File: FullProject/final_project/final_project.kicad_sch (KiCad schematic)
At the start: 46 parts, among them J1 Conn_WallSocket, J2 Weight Sensor Connector, J3 PIR Array Connector 01, J4 PIR Array Connector 02, J5 PIR Array Connector 03, J6 pH Sensor Connector, J7 Keypad Connector, J8 LCD Connector, J9 Conn_01x02_Female, M1 Motor_DC, M2 Motor_Servo, Q1 2N4403, U1 L7805, U2 LM7809_TO220, U3 LM7812_TO220, U4 ATmega32A-P, U5 L293D, U6 SIM900, U7 DS3232M, U8 PCF8574

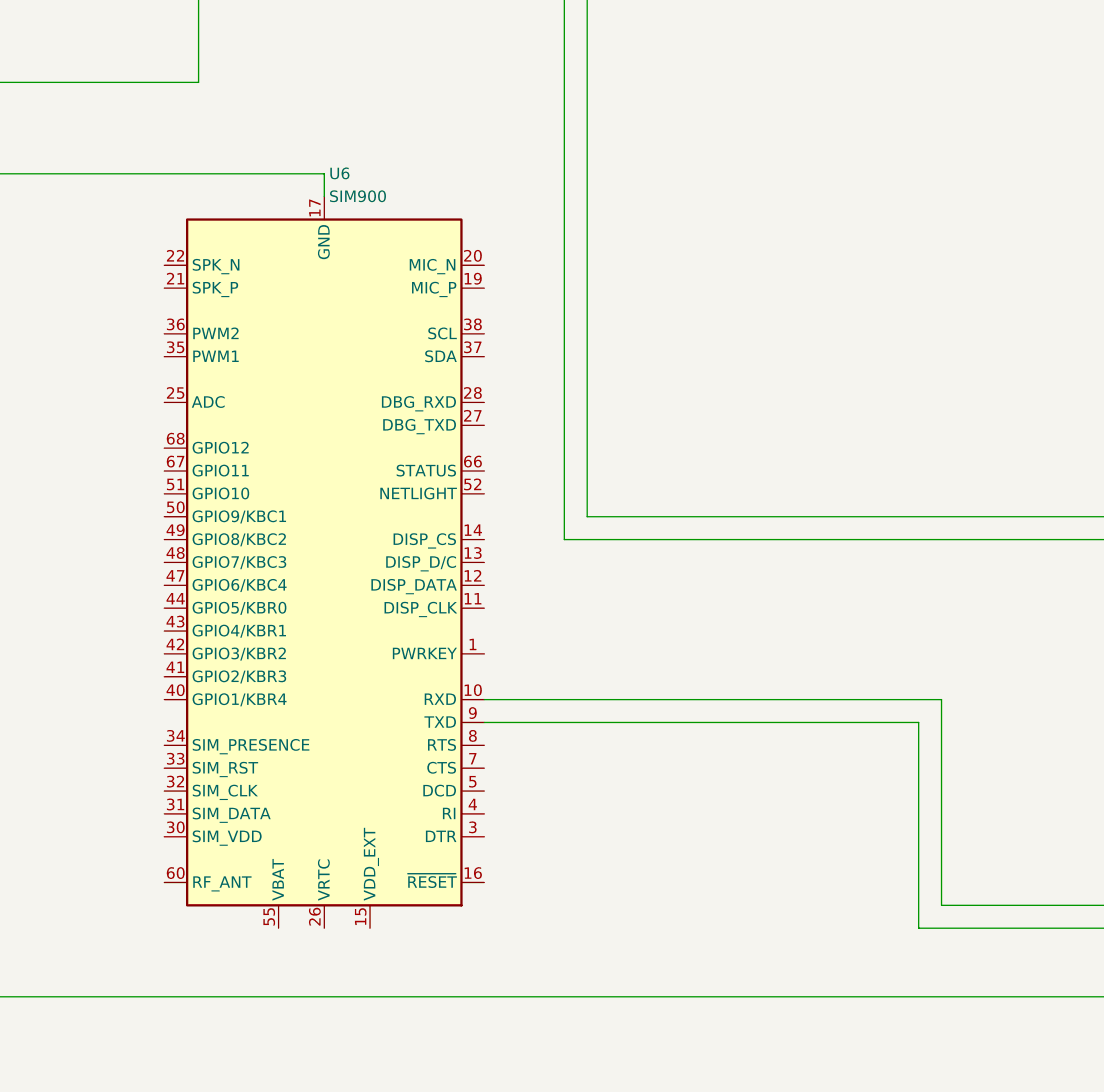
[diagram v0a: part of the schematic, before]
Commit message: add
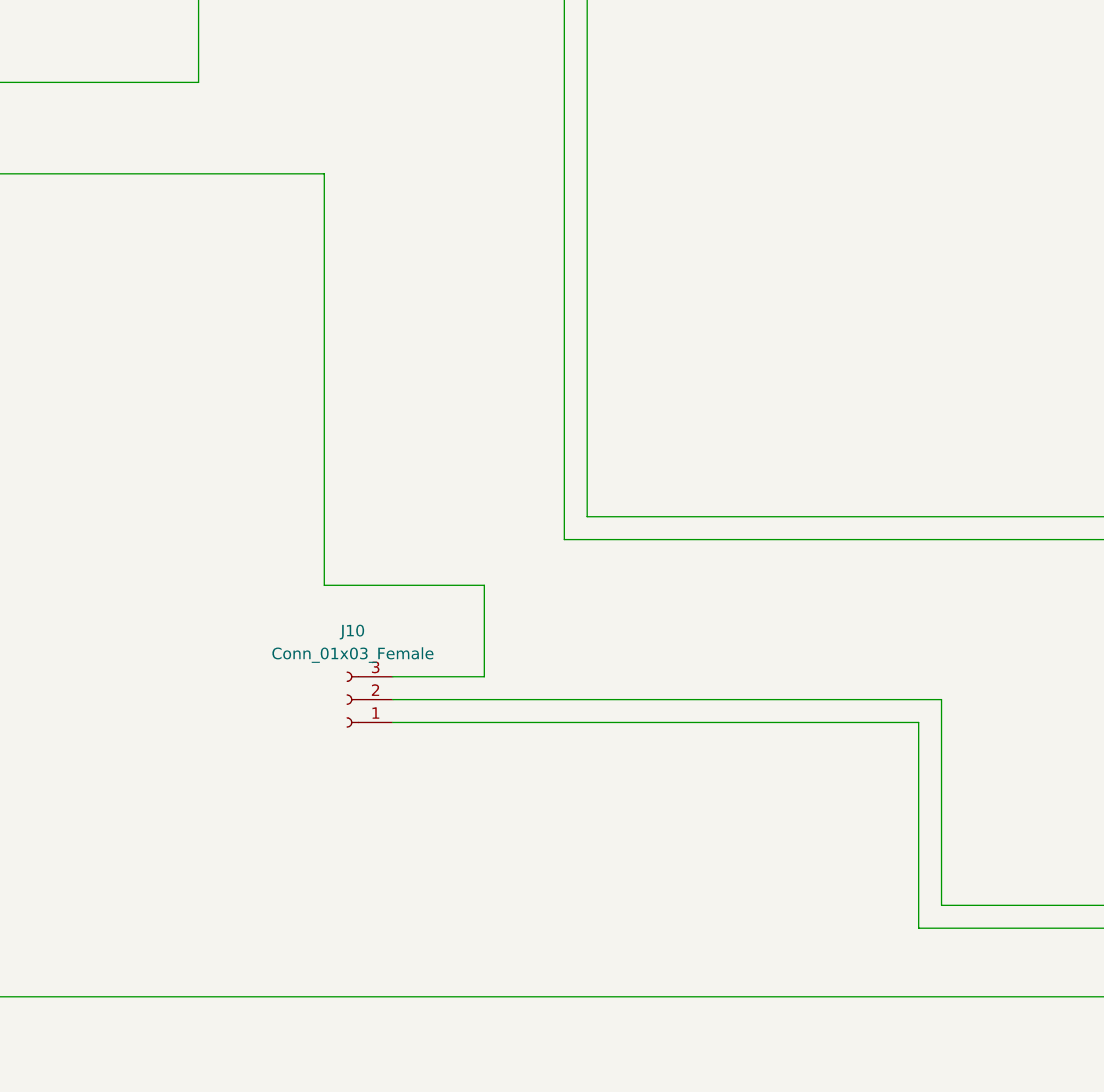
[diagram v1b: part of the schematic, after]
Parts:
- removed U6: SIM900, RF_GSM:SIMCom_SIM900, symbol RF_GSM:SIM900
- added J10: Conn_01x03_Female, Connector_PinSocket_2.54mm:PinSocket_1x03_P2.54mm_Vertical, symbol Connector:Conn_01x03_Female
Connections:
- net at BZ1.2 (+), C1.2, C2.1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: now also J10.3 (Pin_3)
- net at U4.15 (PD1): now also J10.2 (Pin_2)
- net at U4.14 (PD0): now also J10.1 (Pin_1)
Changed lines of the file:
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@@
     (stroke (width 0) (type default) (color 0 0 0 0))
   )
-  (wire (pts (xy 104.14 186.69) (xy 152.4 186.69))
+  (wire (pts (xy 93.98 186.69) (xy 152.4 186.69))
     (stroke (width 0) (type default) (color 0 0 0 0))
   )
@@
     (stroke (width 0) (type default) (color 0 0 0 0))
   )
-  (wire (pts (xy 104.14 184.15) (xy 154.94 184.15))
+  (wire (pts (xy 93.98 184.15) (xy 154.94 184.15))
     (stroke (width 0) (type default) (color 0 0 0 0))
   )
@@
     (stroke (width 0) (type default) (color 0 0 0 0))
   )
+  (wire (pts (xy 104.14 181.61) (xy 93.98 181.61))
+    (stroke (width 0) (type default) (color 0 0 0 0))
+  )
   (wire (pts (xy 113.03 166.37) (xy 175.26 166.37))
     (stroke (width 0) (type default) (color 0 0 0 0))
@@
     (stroke (width 0) (type default) (color 0 0 0 0))
   )
-  (wire (pts (xy 86.36 125.73) (xy 86.36 128.27))
-    (stroke (width 0) (type default) (color 0 0 0 0))
-  )
   (wire (pts (xy 234.95 184.15) (xy 228.6 184.15))
     (stroke (width 0) (type default) (color 0 0 0 0))
@@
     (stroke (width 0) (type default) (color 0 0 0 0))
   )
+  (wire (pts (xy 86.36 125.73) (xy 86.36 171.45))
+    (stroke (width 0) (type default) (color 0 0 0 0))
+  )
   (wire (pts (xy 292.1 224.79) (xy 248.92 224.79))
     (stroke (width 0) (type default) (color 0 0 0 0))
@@
     (stroke (width 0) (type default) (color 0 0 0 0))
   )
+  (wire (pts (xy 86.36 171.45) (xy 104.14 171.45))
+    (stroke (width 0) (type default) (color 0 0 0 0))
+  )
   (wire (pts (xy 241.3 280.67) (xy 241.3 276.86))
     (stroke (width 0) (type default) (color 0 0 0 0))
@@
   )
   (wire (pts (xy 76.2 59.69) (xy 72.39 59.69))
+    (stroke (width 0) (type default) (color 0 0 0 0))
+  )
+  (wire (pts (xy 104.14 171.45) (xy 104.14 181.61))
     (stroke (width 0) (type default) (color 0 0 0 0))
   )
@@
     (pin "1")
     (pin "2")
-  )
-  (symbol (lib_id "RF_GSM:SIM900") (at 86.36 168.91 180) (unit 1)
-    (in_bom yes) (on_board yes) (fields_autoplaced)
-    (property "Reference" "U6" (id 0) (at 86.8806 125.73 0)
-      (effects (font (size 1.27 1.27)) (justify right))
-    )
-    (property "Value" "SIM900" (id 1) (at 86.8806 128.27 0)
-      (effects (font (size 1.27 1.27)) (justify right))
-    )
-    (property "Footprint" "RF_GSM:SIMCom_SIM900" (id 2) (at 73.66 129.54 0)
-      (effects (font (size 1.27 1.27)) hide)
-    )
-    (property "Datasheet" "http://simcom.ee/documents/SIM900/SIM900_Hardware%20Design_V2.05.pdf" (id 3) (at 137.16 201.93 0)
-      (effects (font (size 1.27 1.27)) hide)
-    )
-    (pin "1")
-    (pin "10")
-    (pin "11")
-    (pin "12")
-    (pin "13")
-    (pin "14")
-    (pin "15")
-    (pin "16")
-    (pin "17")
-    (pin "18")
-    (pin "19")
-    (pin "2")
-    (pin "20")
-    (pin "21")
-    (pin "22")
-    (pin "23")
-    (pin "24")
-    (pin "25")
-    (pin "26")
-    (pin "27")
-    (pin "28")
-    (pin "29")
-    (pin "3")
-    (pin "30")
-    (pin "31")
-    (pin "32")
-    (pin "33")
-    (pin "34")
-    (pin "35")
-    (pin "36")
-    (pin "37")
-    (pin "38")
-    (pin "39")
-    (pin "4")
-    (pin "40")
-    (pin "41")
-    (pin "42")
-    (pin "43")
-    (pin "44")
-    (pin "45")
-    (pin "46")
-    (pin "47")
-    (pin "48")
-    (pin "49")
-    (pin "5")
-    (pin "50")
-    (pin "51")
-    (pin "52")
-    (pin "53")
-    (pin "54")
-    (pin "55")
-    (pin "56")
-    (pin "57")
-    (pin "58")
-    (pin "59")
-    (pin "6")
-    (pin "60")
-    (pin "61")
-    (pin "62")
-    (pin "63")
-    (pin "64")
-    (pin "65")
-    (pin "66")
-    (pin "67")
-    (pin "68")
-    (pin "7")
-    (pin "8")
-    (pin "9")
   )
   (symbol (lib_id "Device:Buzzer") (at 384.81 22.86 90) (unit 1)
@@
     (pin "9")
   )
+  (symbol (lib_id "Connector:Conn_01x03_Female") (at 88.9 184.15 180) (unit 1)
+    (in_bom yes) (on_board yes) (fields_autoplaced)
+    (property "Reference" "J10" (id 0) (at 89.535 176.53 0))
+    (property "Value" "Conn_01x03_Female" (id 1) (at 89.535 179.07 0))
+    (property "Footprint" "Connector_PinSocket_2.54mm:PinSocket_1x03_P2.54mm_Vertical" (id 2) (at 88.9 184.15 0)
+      (effects (font (size 1.27 1.27)) hide)
+    )
+    (property "Datasheet" "~" (id 3) (at 88.9 184.15 0)
+      (effects (font (size 1.27 1.27)) hide)
+    )
+    (pin "1")
+    (pin "2")
+    (pin "3")
+  )
   (symbol (lib_id "Connector:Conn_01x04_Female") (at 162.56 21.59 90) (unit 1)
     (in_bom yes) (on_board yes) (fields_autoplaced)
@@
       (reference "J9") (unit 1) (value "Conn_01x02_Female") (footprint "Connector_Phoenix_MSTB:PhoenixContact_MSTBA_2,5_2-G_1x02_P5.00mm_Horizontal")
     )
+    (path "/baf87e68-222c-4493-8e04-3522cc8ab4bc"
+      (reference "J10") (unit 1) (value "Conn_01x03_Female") (footprint "Connector_PinSocket_2.54mm:PinSocket_1x03_P2.54mm_Vertical")
+    )
     (path "/0c9bf32b-4a6c-4391-8a56-38b7d9d09a1c"
       (reference "L1") (unit 1) (value "INDUCTOR") (footprint "Inductor_THT:L_Axial_L9.5mm_D4.0mm_P12.70mm_Horizontal_Fastron_SMCC")
@@
       (reference "U5") (unit 1) (value "L293D") (footprint "Package_DIP:DIP-16_W7.62mm")
     )
-    (path "/96b4594b-45d0-43eb-9b71-f49b45775003"
-      (reference "U6") (unit 1) (value "SIM900") (footprint "RF_GSM:SIMCom_SIM900")
-    )
     (path "/015fffda-3137-49f0-8b5a-b64c080b9a7f"
